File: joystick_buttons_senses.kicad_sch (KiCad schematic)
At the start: 73 parts, among them J3 Joystick, J4 Micro_SD, Q1 2N2907, Q2 2N2907, SW1 A, SW2 B, SW3 X, SW4 Y, SW5 L, SW6 R, U10 LM61, U5 24LC512, U6 23KXX, U7 74HC4051, U8 MMA8452Q, U9 SST26VF032B

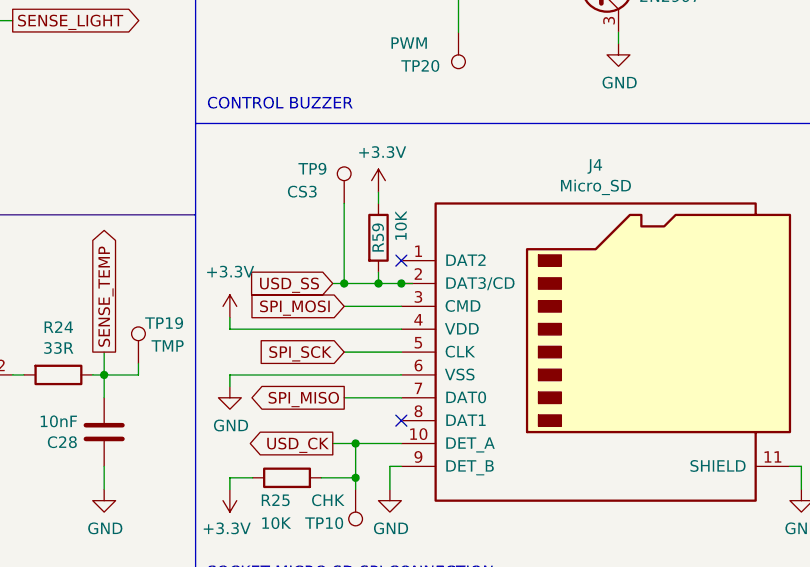
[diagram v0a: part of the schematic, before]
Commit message: 26/12/13/A
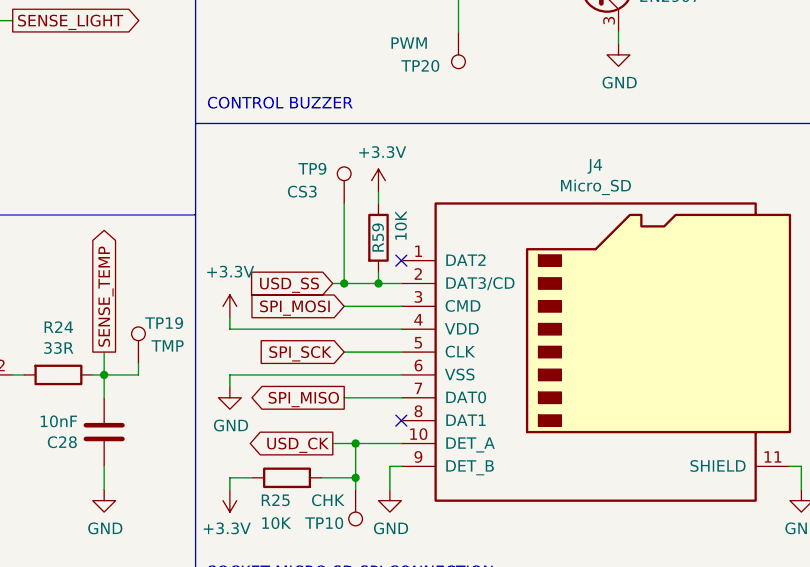
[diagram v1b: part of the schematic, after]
